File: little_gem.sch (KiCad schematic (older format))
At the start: 12 parts, among them J1 AudioPlug2, J2 Conn_01x02_Female, U1 LM386

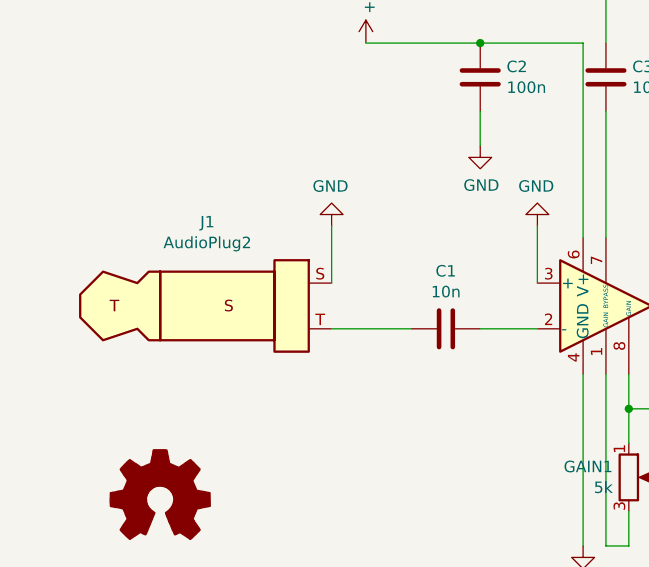
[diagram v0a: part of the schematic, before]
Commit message: Fixed footprints
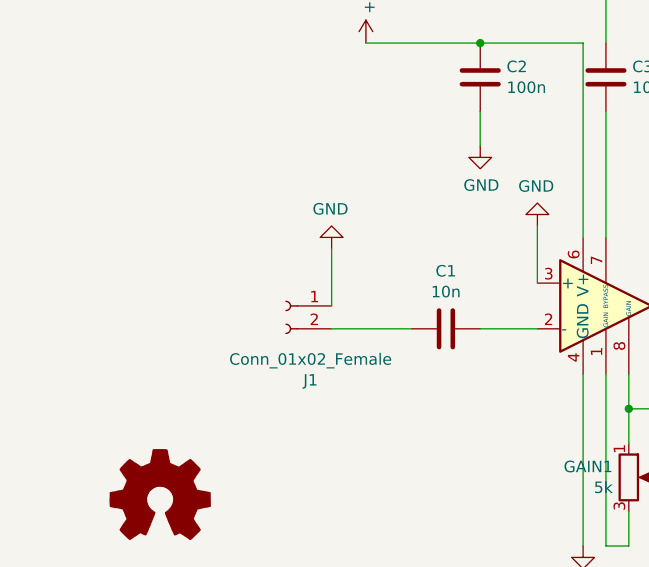
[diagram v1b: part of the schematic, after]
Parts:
- removed J1: AudioPlug2, Connector_PinHeader_2.00mm:PinHeader_1x02_P2.00mm_Vertical_LittleGem, symbol Connector:AudioPlug2
- added J1: Conn_01x02_Female, Connector_PinHeader_2.54mm:PinHeader_1x02_P2.54mm_Vertical, symbol Connector:Conn_01x02_Female
- LS1: footprint Connector_PinHeader_2.00mm:PinHeader_1x02_P2.00mm_Vertical -> Connector_PinHeader_2.54mm:PinHeader_1x02_P2.54mm_Vertical
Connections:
- net GND: now also J1.1 (Pin_1)
- net at C1.2: now also J1.2 (Pin_2)
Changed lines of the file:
@@
 	4700 3550 4700 3800
 Wire Wire Line
-	3800 3550 3800 3800
+	3800 3650 3800 3900
 Wire Wire Line
 	4450 3200 4450 3050
@@
 L power:GND #PWR01
 U 1 1 5EF4EC5F
-P 3800 3550
-F 0 "#PWR01" H 3800 3300 50  0001 C CNN
-F 1 "GND" H 3805 3377 50  0000 C CNN
-F 2 "" H 3800 3550 50  0001 C CNN
-F 3 "" H 3800 3550 50  0001 C CNN
-	1    3800 3550
+P 3800 3650
+F 0 "#PWR01" H 3800 3400 50  0001 C CNN
+F 1 "GND" H 3805 3477 50  0000 C CNN
+F 2 "" H 3800 3650 50  0001 C CNN
+F 3 "" H 3800 3650 50  0001 C CNN
+	1    3800 3650
 	-1   0    0    1
 $EndComp
@@
 $EndComp
 $Comp
-L Connector:AudioPlug2 J1
-U 1 1 5EF095AF
-P 3200 3900
-F 0 "J1" H 3257 4267 50  0000 C CNN
-F 1 "AudioPlug2" H 3257 4176 50  0000 C CNN
-F 2 "Connector_PinHeader_2.00mm:PinHeader_1x02_P2.00mm_Vertical_LittleGem" H 3550 3850 50  0001 C CNN
-F 3 "~" H 3550 3850 50  0001 C CNN
-	1    3200 3900
-	1    0    0    -1
-$EndComp
-$Comp
 L Device:Speaker LS1
 U 1 1 5EF184C9
@@
 F 0 "LS1" H 7370 4346 50  0000 L CNN
 F 1 "Speaker" H 7370 4255 50  0000 L CNN
-F 2 "Connector_PinHeader_2.00mm:PinHeader_1x02_P2.00mm_Vertical" H 7200 4150 50  0001 C CNN
+F 2 "Connector_PinHeader_2.54mm:PinHeader_1x02_P2.54mm_Vertical" H 7200 4150 50  0001 C CNN
 F 3 "~" H 7190 4300 50  0001 C CNN
 	1    7200 4350
@@
 Wire Wire Line
 	2950 2150 2950 2350
+$Comp
+L Connector:Conn_01x02_Female J1
+U 1 1 5F4FF7F7
+P 3600 3900
+F 0 "J1" H 3492 3575 50  0000 C CNN
+F 1 "Conn_01x02_Female" H 3492 3666 50  0000 C CNN
+F 2 "Connector_PinHeader_2.54mm:PinHeader_1x02_P2.54mm_Vertical" H 3600 3900 50  0001 C CNN
+F 3 "~" H 3600 3900 50  0001 C CNN
+	1    3600 3900
+	-1   0    0    -1
+$EndComp
 $EndSCHEMATC
